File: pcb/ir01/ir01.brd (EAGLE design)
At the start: 65 x 30.5 mm, 9 parts

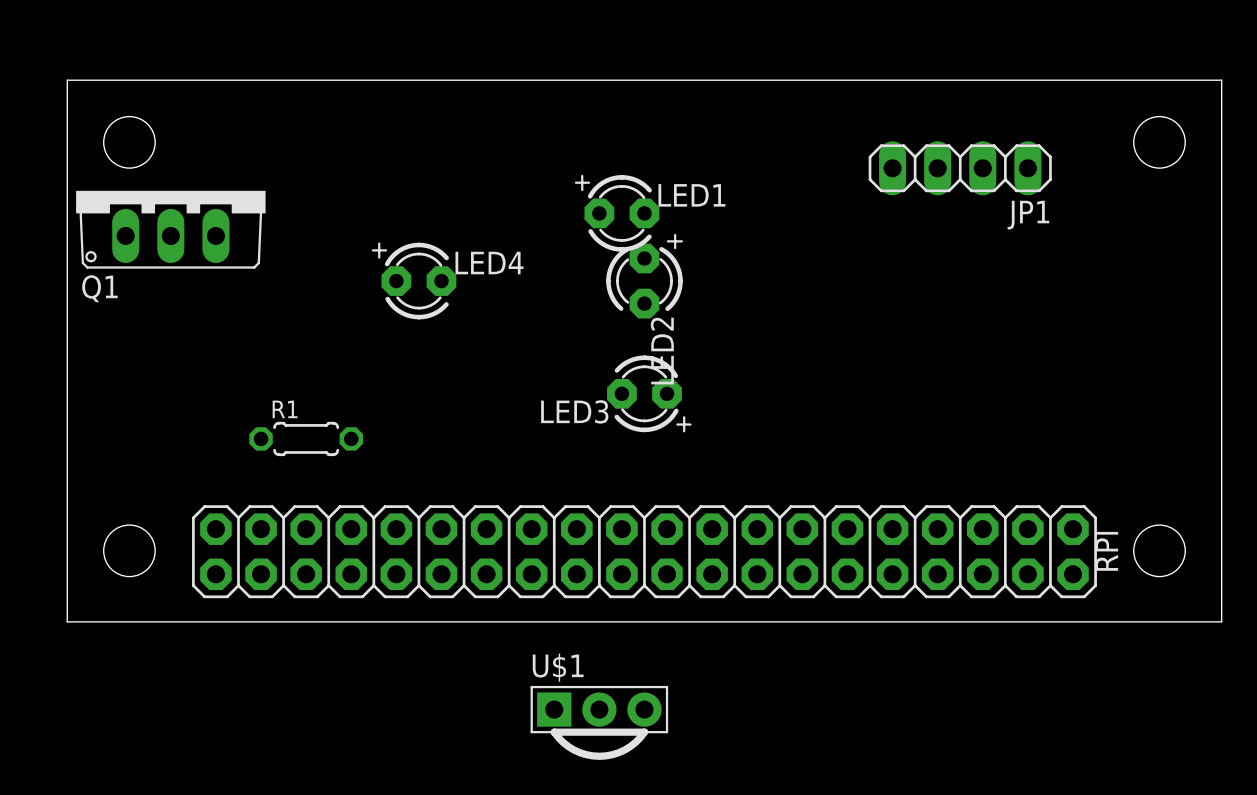
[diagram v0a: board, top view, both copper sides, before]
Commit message: update
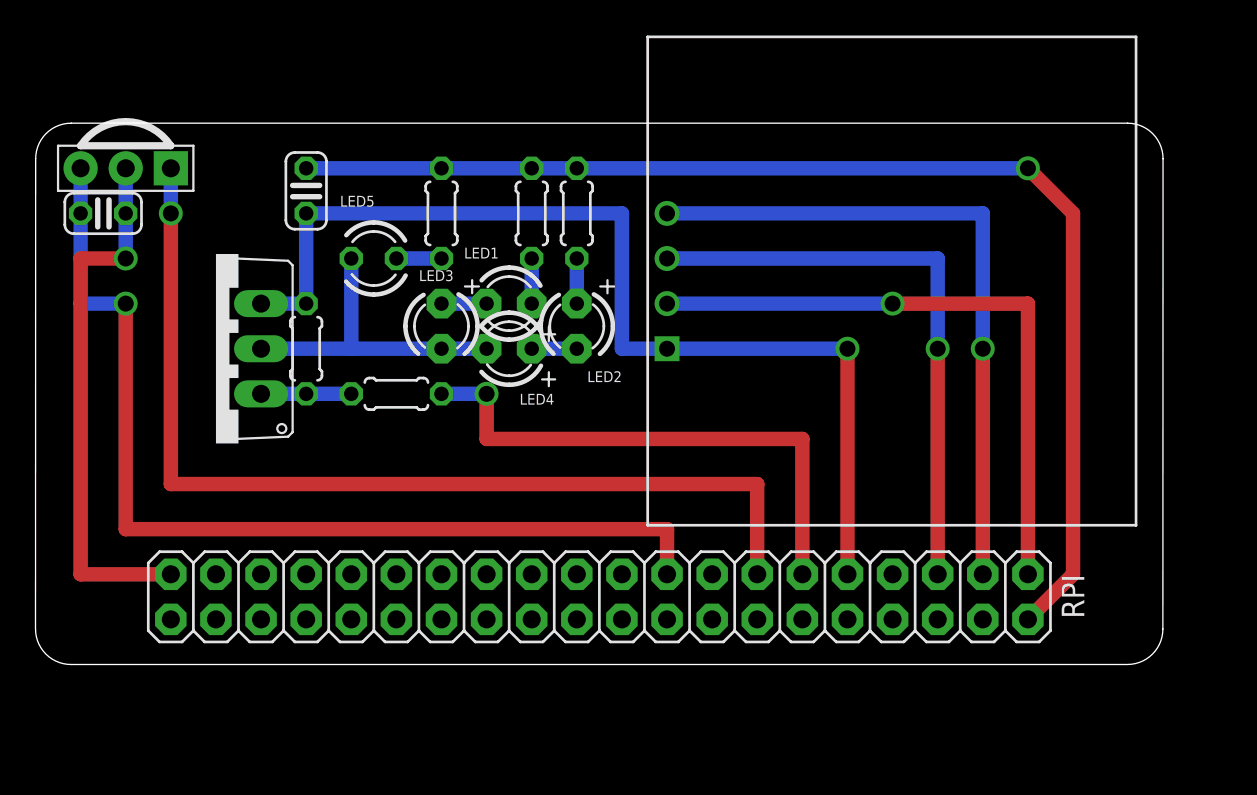
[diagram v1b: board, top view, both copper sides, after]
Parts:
- removed JP1: (no value), pinhead:1X04
- added C1: 0.1μF(104), rcl:C025-024X044
- added C2: 47μF, rcl:C025-024X044
- added LED5: (no value), led:LED3MM
- added OLED: OLED-SSD1306-0.96, ytani1:OLED-I2C-0.96
- added R2: 10ｋΩ, rcl:0204/5
- added R3, R4: 10Ω, rcl:0204/5
- added R5: 1KΩ, rcl:0204/5
- Q1: value (none) -> 2SK4033
- R1: value (none) -> 330Ω
- moved U$1 40.5 mm to (5.08, 27.9), turned to 180 degrees
- moved LED3 12.0 mm to (22.9, 19.1), turned to 270 degrees
- moved Q1 9.25 mm to (10.2, 17.8), turned to 90 degrees
- moved LED1 8.13 mm to (26.7, 20.3), turned to 180 degrees
- moved LED4 6.35 mm to (26.7, 17.8), turned to 180 degrees
- moved R1 5.68 mm to (20.3, 15.2), turned to 180 degrees
- moved LED2 4.58 mm to (30.5, 19.1)
- moved RPI 3.59 mm to (31.8, 3.81)
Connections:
- removed net N$1: JP1.1, RPI.1, RPI.17
- removed net N$2: JP1.2, RPI.3
- removed net N$3: JP1.3, RPI.5
- removed net N$6: RPI.2, RPI.4
- removed net VCC: U$1.3
- new net +3V3A: OLED.VCC, RPI.1
- new net +3V3B: C1.1, RPI.17, U$1.3
- new net +5V: C2.1, R3.2, R4.2, R5.2, RPI.2
- new net IRIN: RPI.13, U$1.1
- new net IROUT: R1.1, RPI.11
- new net IROUT2: Q1.1, R1.2, R2.2
- new net LEDIN0: LED5.A, R5.1
- new net LEDIN1: LED2.A, R3.1
- new net LEDIN2: LED1.A, R4.1
- new net N$5: LED2.K, LED4.A
- new net N$7: LED1.K, LED3.A
- new net Q1IN: LED3.K, LED4.K, LED5.K, Q1.2
- new net SCL: OLED.SCL, RPI.5
- new net SDA: OLED.SDA, RPI.3
- net GND: now also C1.2, C2.2, OLED.GND, Q1.3, R2.1; no longer JP1.4, RPI.14, RPI.20, RPI.25, RPI.30, RPI.34, RPI.6
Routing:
- net GND: track 0.00 -> 88.9 mm, vias 0 -> 2
- net +5V: track 0.00 -> 68.1 mm, vias 0 -> 1
- net +3V3B: track 0.00 -> 55.9 mm, vias 0 -> 1
- net IRIN: track 0.00 -> 55.9 mm, vias 0 -> 1
- net SDA: track 0.00 -> 38.1 mm, vias 0 -> 1
- net +3V3A: track 0.00 -> 35.6 mm, vias 0 -> 1
- net SCL: track 0.00 -> 33.0 mm, vias 0 -> 1
- net IROUT: track 0.00 -> 30.5 mm, vias 0 -> 1
- net Q1IN: track 0.00 -> 17.8 mm
- net IROUT2: track 0.00 -> 5.08 mm
- net N$7: track 0.00 -> 2.54 mm
- net N$5: track 0.00 -> 2.54 mm
- net LEDIN2: track 0.00 -> 2.54 mm
- net LEDIN1: track 0.00 -> 2.54 mm
- net LEDIN0: track 0.00 -> 2.54 mm
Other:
- board size 65 x 30.5 mm -> 63.5 x 30.5 mm
